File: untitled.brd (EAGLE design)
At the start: 34.6 x 34.6 mm, 11 parts, among them IC1 ATTINY13-20PU, SW1 1825910-6

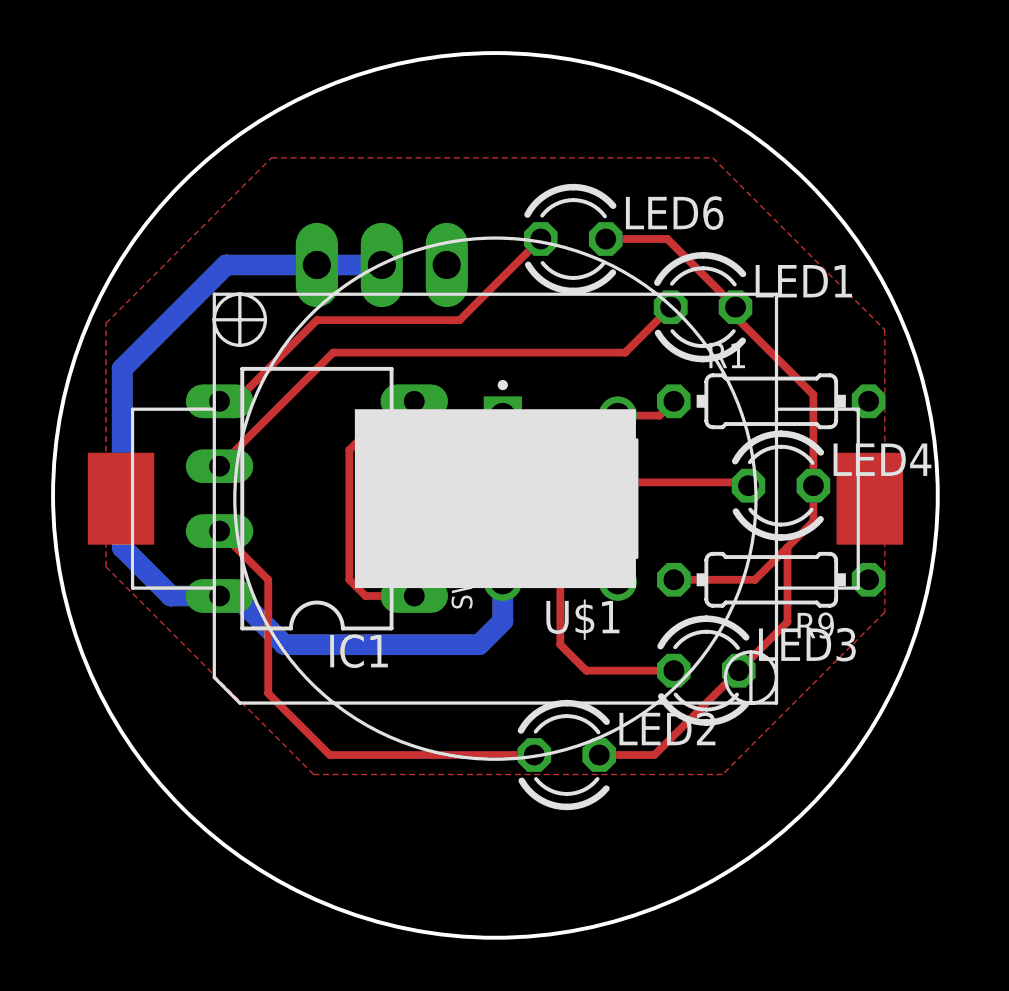
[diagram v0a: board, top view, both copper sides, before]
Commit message: errors fixed
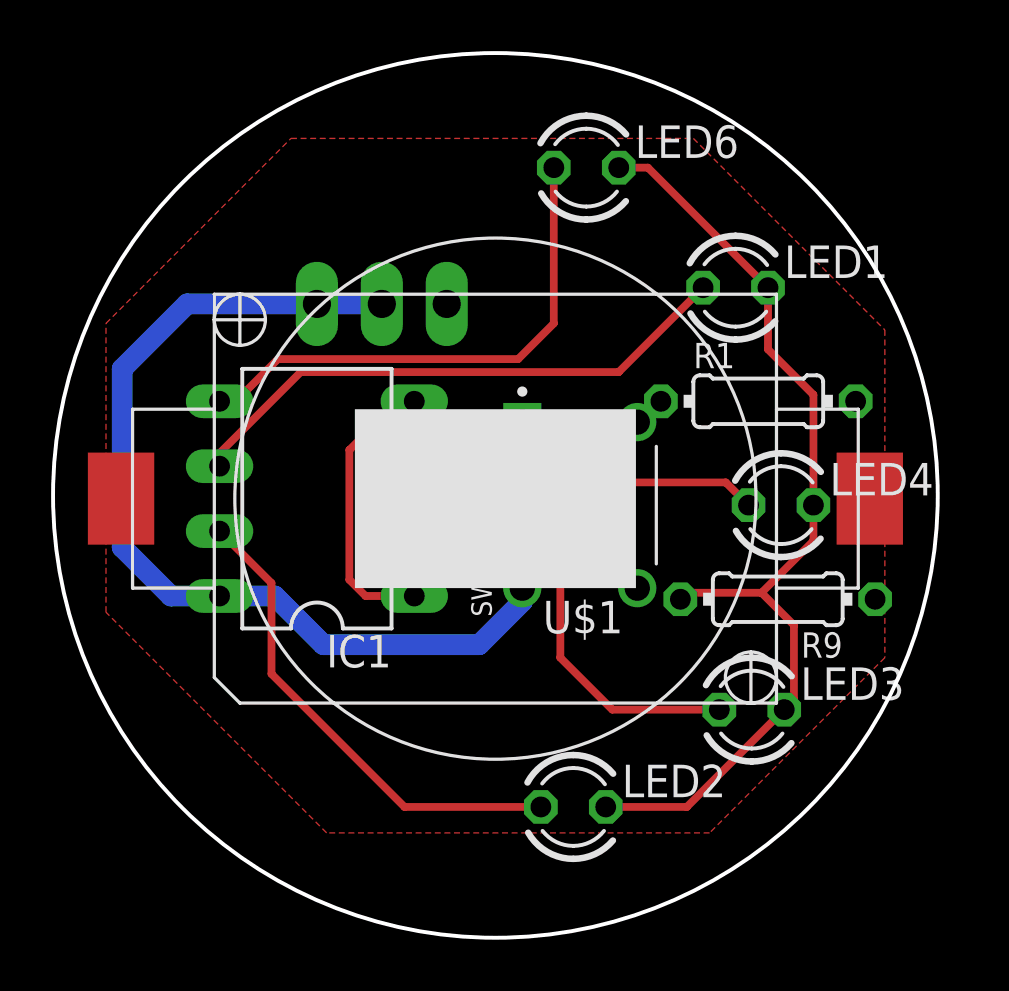
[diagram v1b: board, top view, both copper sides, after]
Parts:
- moved LED6 2.84 mm to (95.0, 73.3)
- moved LED3 2.34 mm to (101.5, 52.1)
- moved LED2 2.05 mm to (94.5, 48.3)
- moved S2 1.52 mm to (87.0, 67.9)
- moved LED1 1.48 mm to (100.8, 68.6)
- moved R9 0.80 mm to (102.5, 56.4)
- moved SW1 0.80 mm to (94.7, 60.1)
- moved LED4 0.76 mm to (102.6, 60.1)
- moved R1 0.51 mm to (101.7, 64.1)
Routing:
- net N$1: track 15.2 -> 20.4 mm
- net N$6: track 34.7 -> 38.6 mm
- net N$4: track 14.3 -> 17.0 mm
- net N$2: track 20.2 -> 22.1 mm
- net N$8: track 2.43 -> 1.26 mm
- net N$7: track 14.4 -> 15.1 mm
- net N$3: track 18.6 -> 19.1 mm
- net VCC: track 37.2 -> 36.7 mm
